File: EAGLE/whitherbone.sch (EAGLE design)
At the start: 194 parts, among them IC12 TPS2051BDGN, IC13 SN74AUC1G74, IC14 TPD4S012DRY, IC15 TPD4S012DRY, IC17 SN74LVC2G241DCUR, IC2 SN74LVC1G07DCK, IC4 7805T, IC7 IP4283CZ10-TBR, IC8 IP4283CZ10-TBR, IC9 TDA19988BHN/C1,557, J1 1-1747981-1, Q2 32.768kHz, Q4 24 MHz, T1 BSS138W-7-F, T3 BSS138W-7-F, T4 BSS138W-7-F, U1 OSD3358-512M-BSM, U2 A3967SLBTR, X2 SCHA5B0200, X4 10118192-0001LF

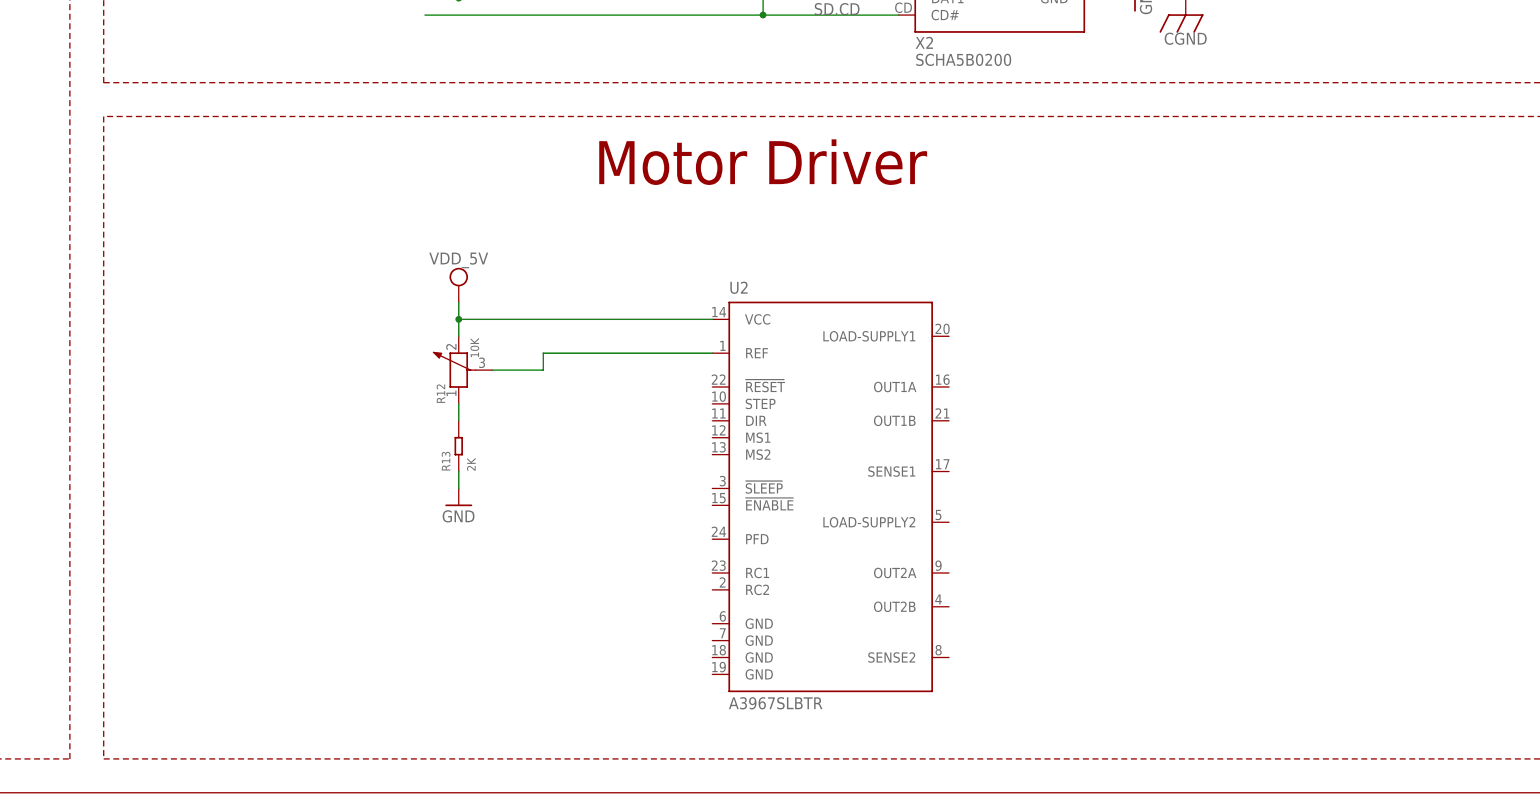
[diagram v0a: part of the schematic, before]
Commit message: Copied BigEasyDriver
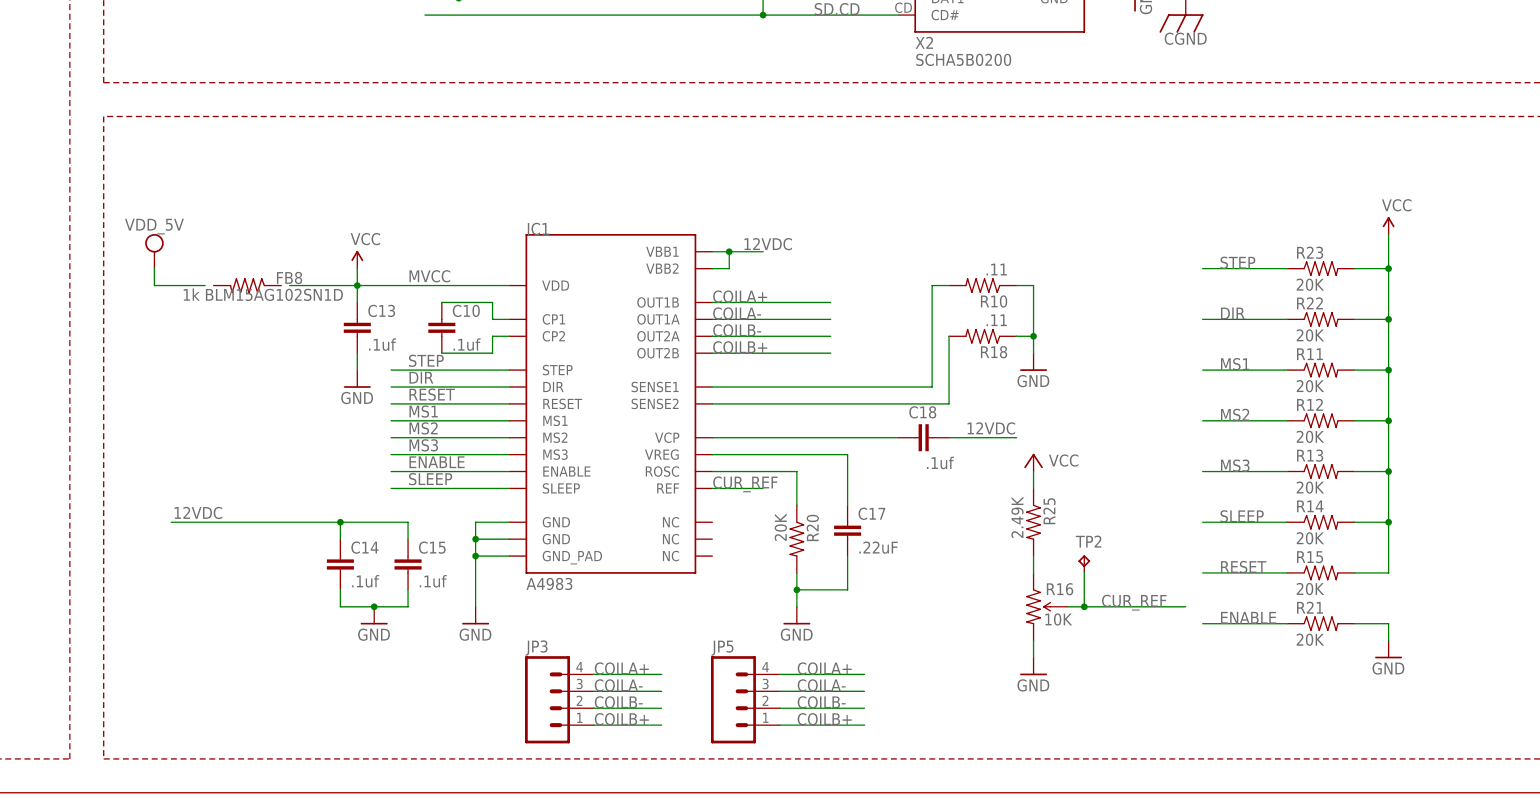
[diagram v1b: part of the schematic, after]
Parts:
- removed U2: A3967SLBTR, A3967SLBTR:A3967SLBTR
- added C10, C13, C14, C15, C18: .1uf, SparkFun:CAP0402-CAP
- added C17: .22uF, SparkFun:CAP0402-CAP
- added FB8: 1k BLM15AG102SN1D, rcl:R-US_R0402
- added IC1: A4983, SparkFun:A4983
- added JP3: (no value), SparkFun:M04PTH
- added JP5: (no value), BigEasyDriver_v11:M04SCREW_LOCK
- added R10, R18: .11, SparkFun:RESISTOR2010
- added R11, R14, R15, R20, R21, R22, R23: 20K, SparkFun:RESISTOR0402-RES
- added R16: 10K, SparkFun:TRIMPOTSMD
- added R25: 2.49K, SparkFun:RESISTOR0402-RES
- added TP2: TPPAD1-13, testpad:TPPAD1-13
- R12: value 10K -> 20K; device Seeed-Resistor:DIP-VR-TOP-ADJ-10K(3P-9.5X9.5X5MM) -> SparkFun:RESISTOR0402-RES
- R13: value 2K -> 20K; device Seeed-Resistor:SMD-RES-2K-1%-1/10W(0603) -> SparkFun:RESISTOR0402-RES
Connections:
- new net COILA+: IC1.OUT1B, JP3.4, JP5.4
- new net COILA-: IC1.OUT1A, JP3.3, JP5.3
- new net COILB+: IC1.OUT2B, JP3.1, JP5.1
- new net COILB-: IC1.OUT2A, JP3.2, JP5.2
- new net CUR_REF: IC1.REF, R16.WIPER, TP2.TP
- new net DIR: IC1.DIR, R22.1
- new net ENABLE: IC1.ENABLE, R21.1
- new net MS1: IC1.MS1, R11.1
- new net MS2: IC1.MS2, R12.1
- new net MS3: IC1.MS3, R13.1
- new net MVCC: C13.1, IC1.VDD, R11.2, R12.2, R13.2, R14.2, R15.2, R22.2, R23.2, R25.1
- new net N$30: IC1.ROSC, R20.1
- new net N$32: IC1.SENSE1, R10.2
- new net N$46: C17.1, IC1.VREG
- new net N$47: C18.1, IC1.VCP
- new net N$48: R16.CCW, R25.2
- new net N$9: C10.1, IC1.CP1
- new net RESET: IC1.RESET, R15.1
- new net SLEEP: IC1.SLEEP, R14.1
- new net STEP: IC1.STEP, R23.1
- net 12VDC: now also C14.1, C15.1, C18.2, IC1.VBB1, IC1.VBB2
- net GND: now also C13.2, C14.2, C15.2, C17.2, IC1.GND@1, IC1.GND@2, IC1.GND_PAD, R10.1, R16.CW, R18.1, R20.2, R21.2; no longer R13.1
- net N$10: now also C10.2, IC1.CP2; no longer R12.3, U2.REF
- net N$31: now also IC1.SENSE2, R18.2; no longer R12.1, R13.2
- net VDD_5V: no longer R12.2, U2.VCC
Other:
- note added: "Attribution 3.0 US License"
- note added: "BigEasyDriver v1.2 by Brian Schmalz is"
- note added: "Current adj pot"
- note added: "Motor current 0mA to over 2A/phase"
- note added: "licensed under a Creative Commons"
- note added: "www.schmalzhaus.com/BigEasyDriver"
- note removed: "Motor Driver"
